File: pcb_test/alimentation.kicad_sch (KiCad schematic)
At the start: 57 parts, among them Q1 NMOS, Q2 NMOS, U1 TPSM53602RDA, U14 TPS2412D, U15 TPS2412D, U3 TPS74801AWDRC

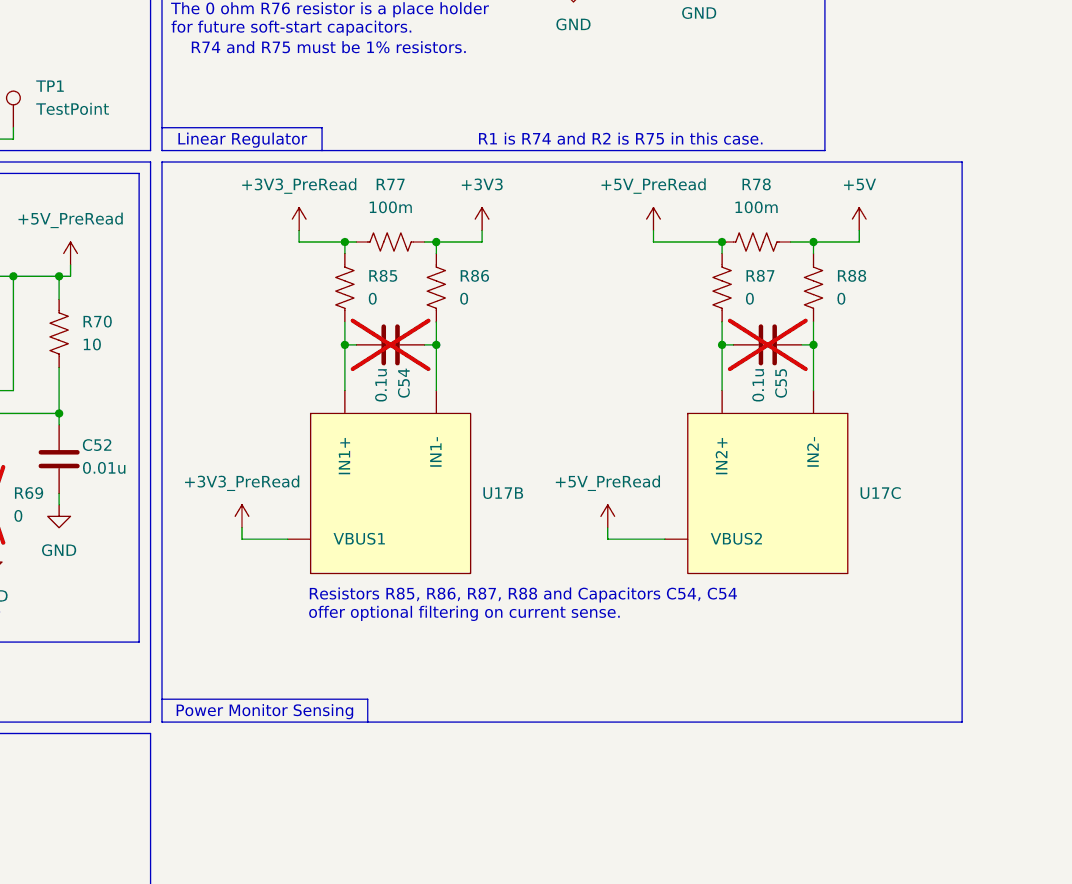
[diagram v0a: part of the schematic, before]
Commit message: Presque fini i guess
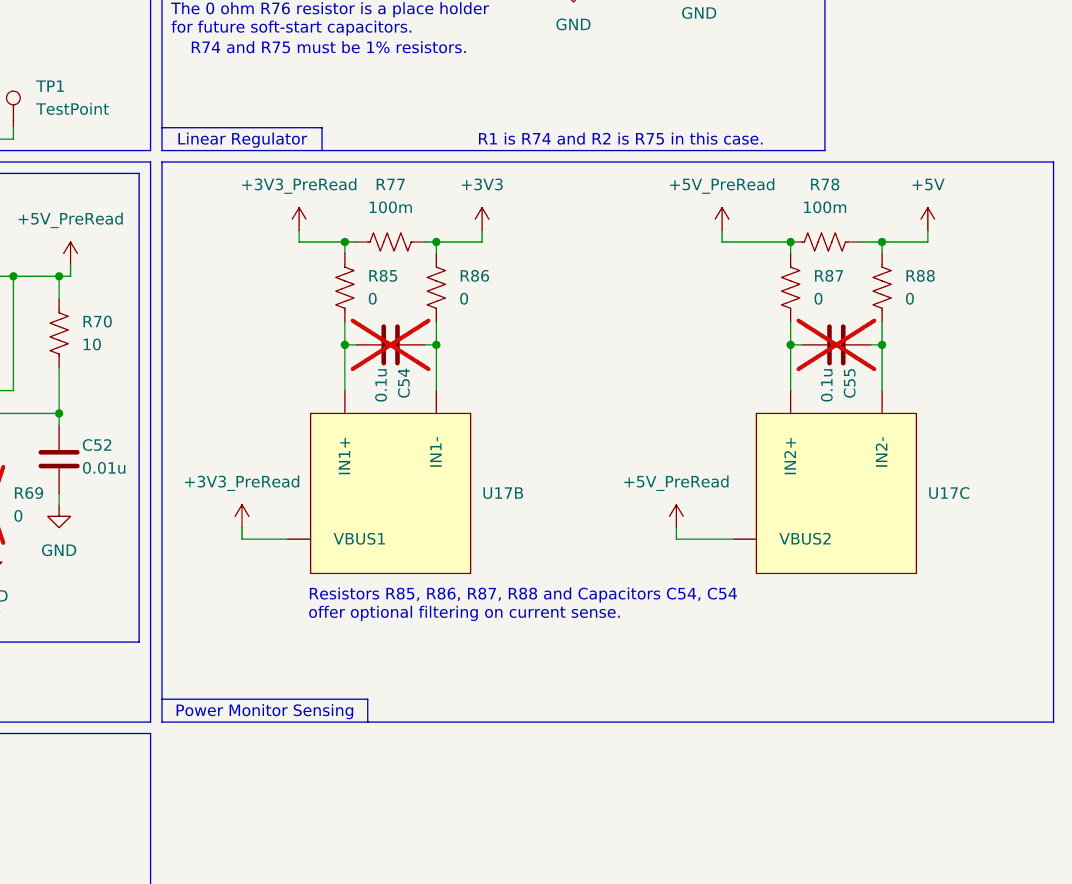
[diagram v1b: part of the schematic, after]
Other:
- moved on the sheet: C55, R78, R87, R88, U17C
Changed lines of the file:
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@@
 	(rectangle
 		(start 142.24 64.77)
-		(end 231.14 127)
+		(end 241.3 127)
 		(stroke
 			(width 0)
@@
 	)
 	(junction
-		(at 204.47 73.66)
+		(at 212.09 73.66)
 		(diameter 0)
 		(color 0 0 0 0)
@@
 	)
 	(junction
-		(at 214.63 73.66)
+		(at 222.25 73.66)
 		(diameter 0)
 		(color 0 0 0 0)
@@
 	)
 	(junction
-		(at 204.47 85.09)
+		(at 212.09 85.09)
 		(diameter 0)
 		(color 0 0 0 0)
@@
 	)
 	(junction
-		(at 214.63 85.09)
+		(at 222.25 85.09)
 		(diameter 0)
 		(color 0 0 0 0)
@@
 	(wire
 		(pts
-			(xy 214.63 73.66) (xy 214.63 74.93)
+			(xy 222.25 73.66) (xy 222.25 74.93)
 		)
 		(stroke
@@
 	(wire
 		(pts
-			(xy 214.63 85.09) (xy 214.63 90.17)
+			(xy 222.25 85.09) (xy 222.25 90.17)
 		)
 		(stroke
@@
 	(wire
 		(pts
-			(xy 219.71 72.39) (xy 219.71 73.66)
+			(xy 227.33 72.39) (xy 227.33 73.66)
 		)
 		(stroke
@@
 	(wire
 		(pts
-			(xy 191.77 105.41) (xy 191.77 106.68)
+			(xy 199.39 105.41) (xy 199.39 106.68)
 		)
 		(stroke
@@
 	(wire
 		(pts
-			(xy 219.71 73.66) (xy 214.63 73.66)
+			(xy 227.33 73.66) (xy 222.25 73.66)
 		)
 		(stroke
@@
 	(wire
 		(pts
-			(xy 212.09 73.66) (xy 214.63 73.66)
+			(xy 219.71 73.66) (xy 222.25 73.66)
 		)
 		(stroke
@@
 	(wire
 		(pts
-			(xy 204.47 85.09) (xy 205.74 85.09)
+			(xy 212.09 85.09) (xy 213.36 85.09)
 		)
 		(stroke
@@
 	(wire
 		(pts
-			(xy 214.63 82.55) (xy 214.63 85.09)
+			(xy 222.25 82.55) (xy 222.25 85.09)
 		)
 		(stroke
@@
 	(wire
 		(pts
-			(xy 204.47 85.09) (xy 204.47 82.55)
+			(xy 212.09 85.09) (xy 212.09 82.55)
 		)
 		(stroke
@@
 	(wire
 		(pts
-			(xy 191.77 106.68) (xy 198.12 106.68)
+			(xy 199.39 106.68) (xy 205.74 106.68)
 		)
 		(stroke
@@
 	(wire
 		(pts
-			(xy 213.36 85.09) (xy 214.63 85.09)
+			(xy 220.98 85.09) (xy 222.25 85.09)
 		)
 		(stroke
@@
 	(wire
 		(pts
-			(xy 196.85 73.66) (xy 204.47 73.66)
+			(xy 204.47 73.66) (xy 212.09 73.66)
 		)
 		(stroke
@@
 	(wire
 		(pts
-			(xy 196.85 72.39) (xy 196.85 73.66)
+			(xy 204.47 72.39) (xy 204.47 73.66)
 		)
 		(stroke
@@
 	(wire
 		(pts
-			(xy 204.47 73.66) (xy 204.47 74.93)
+			(xy 212.09 73.66) (xy 212.09 74.93)
 		)
 		(stroke
@@
 	(wire
 		(pts
-			(xy 204.47 90.17) (xy 204.47 85.09)
+			(xy 212.09 90.17) (xy 212.09 85.09)
 		)
 		(stroke
@@
 	(symbol
 		(lib_id "Device:C")
-		(at 209.55 85.09 270)
+		(at 217.17 85.09 270)
 		(unit 1)
 		(body_style 1)
@@
 		(dnp yes)
 		(property "Reference" "C55"
-			(at 211.074 87.63 0)
+			(at 218.694 87.63 0)
 			(show_name no)
 			(do_not_autoplace no)
@@
 		)
 		(property "Value" "0.1u"
-			(at 208.534 87.63 0)
+			(at 216.154 87.63 0)
 			(show_name no)
 			(do_not_autoplace no)
@@
 		)
 		(property "Footprint" ""
-			(at 205.74 86.0552 0)
+			(at 213.36 86.0552 0)
 			(hide yes)
 			(show_name no)
@@
 		)
 		(property "Datasheet" ""
-			(at 209.55 85.09 0)
+			(at 217.17 85.09 0)
 			(hide yes)
 			(show_name no)
@@
 		)
 		(property "Description" "Unpolarized capacitor"
-			(at 209.55 85.09 0)
+			(at 217.17 85.09 0)
 			(hide yes)
 			(show_name no)
@@
 		(lib_name "INA2227_2")
 		(lib_id "stuff:INA2227")
-		(at 209.55 101.6 0)
+		(at 217.17 101.6 0)
 		(unit 3)
 		(body_style 1)
@@
 		(fields_autoplaced yes)
 		(property "Reference" "U17"
-			(at 219.71 101.5999 0)
+			(at 227.33 101.5999 0)
 			(show_name no)
 			(do_not_autoplace no)
@@
 		)
 		(property "Value" ""
-			(at 209.55 101.6 0)
+			(at 217.17 101.6 0)
 			(show_name no)
 			(do_not_autoplace no)
@@
 		)
 		(property "Footprint" ""
-			(at 209.55 101.6 0)
+			(at 217.17 101.6 0)
 			(hide yes)
 			(show_name no)
@@
 		)
 		(property "Datasheet" ""
-			(at 209.55 101.6 0)
+			(at 217.17 101.6 0)
 			(hide yes)
 			(show_name no)
@@
 		)
 		(property "Description" ""
-			(at 209.55 101.6 0)
+			(at 217.17 101.6 0)
 			(hide yes)
 			(show_name no)
@@
 	(symbol
 		(lib_id "Device:R_US")
-		(at 204.47 78.74 180)
+		(at 212.09 78.74 180)
 		(unit 1)
 		(body_style 1)
@@
 		(fields_autoplaced yes)
 		(property "Reference" "R87"
-			(at 207.01 77.4699 0)
+			(at 214.63 77.4699 0)
 			(show_name no)
 			(do_not_autoplace no)
@@
 		)
 		(property "Value" "0"
-			(at 207.01 80.0099 0)
+			(at 214.63 80.0099 0)
 			(show_name no)
 			(do_not_autoplace no)
@@
 		)
 		(property "Footprint" ""
-			(at 203.454 78.486 90)
+			(at 211.074 78.486 90)
 			(hide yes)
 			(show_name no)
@@
 		)
 		(property "Datasheet" ""
-			(at 204.47 78.74 0)
+			(at 212.09 78.74 0)
 			(hide yes)
 			(show_name no)
@@
 		)
 		(property "Description" "Resistor, US symbol"
-			(at 204.47 78.74 0)
+			(at 212.09 78.74 0)
 			(hide yes)
 			(show_name no)
@@
 	(symbol
 		(lib_id "Device:R_US")
-		(at 208.28 73.66 90)
+		(at 215.9 73.66 90)
 		(unit 1)
 		(body_style 1)
@@
 		(fields_autoplaced yes)
 		(property "Reference" "R78"
-			(at 208.28 67.31 90)
+			(at 215.9 67.31 90)
 			(show_name no)
 			(do_not_autoplace no)
@@
 		)
 		(property "Value" "100m"
-			(at 208.28 69.85 90)
+			(at 215.9 69.85 90)
 			(show_name no)
 			(do_not_autoplace no)
@@
 		)
 		(property "Footprint" ""
-			(at 208.534 72.644 90)
+			(at 216.154 72.644 90)
 			(hide yes)
 			(show_name no)
@@
 		)
 		(property "Datasheet" ""
-			(at 208.28 73.66 0)
+			(at 215.9 73.66 0)
 			(hide yes)
 			(show_name no)
@@
 		)
 		(property "Description" "Resistor, US symbol"
-			(at 208.28 73.66 0)
+			(at 215.9 73.66 0)
 			(hide yes)
 			(show_name no)
@@
 	(symbol
 		(lib_id "Device:R_US")
-		(at 214.63 78.74 180)
+		(at 222.25 78.74 180)
 		(unit 1)
 		(body_style 1)
@@
 		(fields_autoplaced yes)
 		(property "Reference" "R88"
-			(at 217.17 77.4699 0)
+			(at 224.79 77.4699 0)
 			(show_name no)
 			(do_not_autoplace no)
@@
 		)
 		(property "Value" "0"
-			(at 217.17 80.0099 0)
+			(at 224.79 80.0099 0)
 			(show_name no)
 			(do_not_autoplace no)
@@
 		)
 		(property "Footprint" ""
-			(at 213.614 78.486 90)
+			(at 221.234 78.486 90)
 			(hide yes)
 			(show_name no)
@@
 		)
 		(property "Datasheet" ""
-			(at 214.63 78.74 0)
+			(at 222.25 78.74 0)
 			(hide yes)
 			(show_name no)
@@
 		)
 		(property "Description" "Resistor, US symbol"
-			(at 214.63 78.74 0)
+			(at 222.25 78.74 0)
 			(hide yes)
 			(show_name no)
@@
 	(symbol
 		(lib_id "power:+5V")
-		(at 191.77 105.41 0)
+		(at 199.39 105.41 0)
 		(unit 1)
 		(body_style 1)
@@
 		(fields_autoplaced yes)
 		(property "Reference" "#PWR0142"
-			(at 191.77 109.22 0)
+			(at 199.39 109.22 0)
 			(hide yes)
 			(show_name no)
@@
 		)
 		(property "Value" "+5V_PreRead"
-			(at 191.77 100.33 0)
+			(at 199.39 100.33 0)
 			(show_name no)
 			(do_not_autoplace no)
@@
 		)
 		(property "Footprint" ""
-			(at 191.77 105.41 0)
+			(at 199.39 105.41 0)
 			(hide yes)
 			(show_name no)
@@
 		)
 		(property "Datasheet" ""
-			(at 191.77 105.41 0)
+			(at 199.39 105.41 0)
 			(hide yes)
 			(show_name no)
@@
 		)
 		(property "Description" "Power symbol creates a global label with name \"+5V\""
-			(at 191.77 105.41 0)
+			(at 199.39 105.41 0)
 			(hide yes)
 			(show_name no)
@@
 	(symbol
 		(lib_id "power:+5V")
-		(at 196.85 72.39 0)
+		(at 204.47 72.39 0)
 		(unit 1)
 		(body_style 1)
@@
 		(fields_autoplaced yes)
 		(property "Reference" "#PWR0136"
-			(at 196.85 76.2 0)
+			(at 204.47 76.2 0)
 			(hide yes)
 			(show_name no)
@@
 		)
 		(property "Value" "+5V_PreRead"
-			(at 196.85 67.31 0)
+			(at 204.47 67.31 0)
 			(show_name no)
 			(do_not_autoplace no)
@@
 		)
 		(property "Footprint" ""
-			(at 196.85 72.39 0)
+			(at 204.47 72.39 0)
 			(hide yes)
 			(show_name no)
@@
 		)
 		(property "Datasheet" ""
-			(at 196.85 72.39 0)
+			(at 204.47 72.39 0)
 			(hide yes)
 			(show_name no)
@@
 		)
 		(property "Description" "Power symbol creates a global label with name \"+5V\""
-			(at 196.85 72.39 0)
+			(at 204.47 72.39 0)
 			(hide yes)
 			(show_name no)
@@
 	(symbol
 		(lib_id "power:+5V")
-		(at 219.71 72.39 0)
+		(at 227.33 72.39 0)
 		(unit 1)
 		(body_style 1)
@@
 		(fields_autoplaced yes)
 		(property "Reference" "#PWR0137"
-			(at 219.71 76.2 0)
+			(at 227.33 76.2 0)
 			(hide yes)
 			(show_name no)
@@
 		)
 		(property "Value" "+5V"
-			(at 219.71 67.31 0)
+			(at 227.33 67.31 0)
 			(show_name no)
 			(do_not_autoplace no)
@@
 		)
 		(property "Footprint" ""
-			(at 219.71 72.39 0)
+			(at 227.33 72.39 0)
 			(hide yes)
 			(show_name no)
@@
 		)
 		(property "Datasheet" ""
-			(at 219.71 72.39 0)
+			(at 227.33 72.39 0)
 			(hide yes)
 			(show_name no)
@@
 		)
 		(property "Description" "Power symbol creates a global label with name \"+5V\""
-			(at 219.71 72.39 0)
+			(at 227.33 72.39 0)
 			(hide yes)
 			(show_name no)
